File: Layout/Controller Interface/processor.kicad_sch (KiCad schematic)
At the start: 17 parts, among them J1 USB_C_Receptacle_USB2.0, SW2 SW_Push, SW3 SW_Push, SW4 SW_Push, U1 RP2040, U3 W25X40CLSN, Y1 12MHz

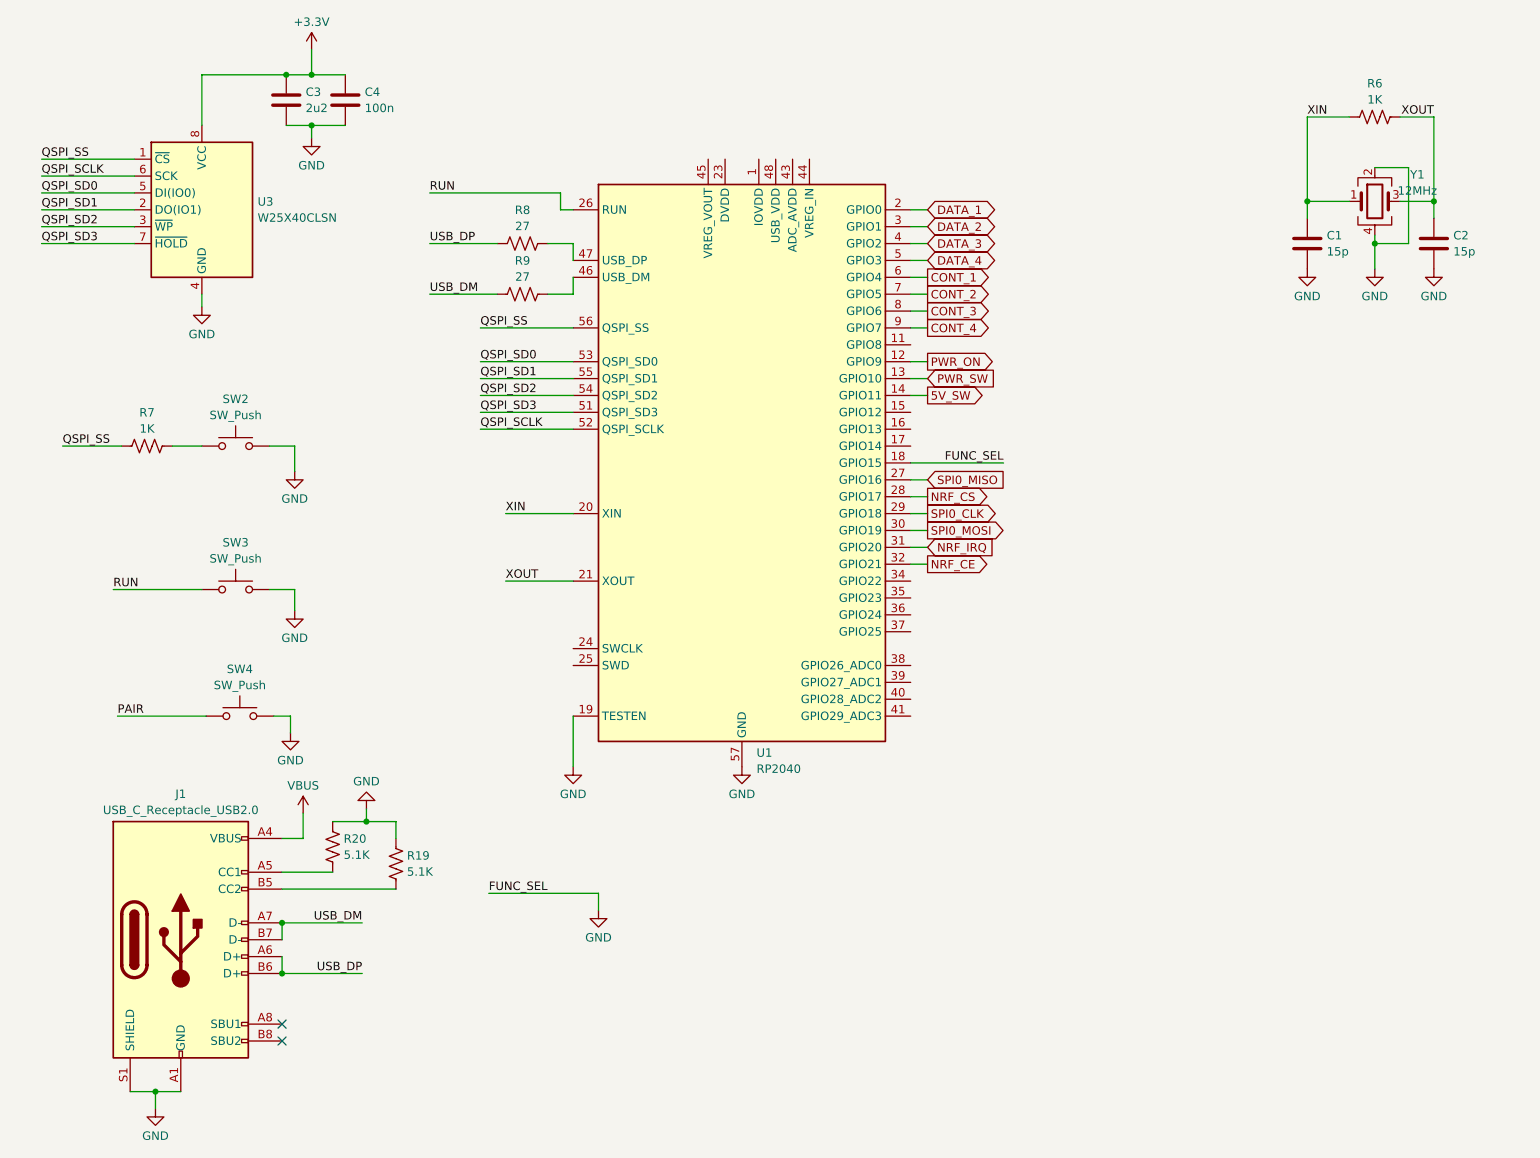
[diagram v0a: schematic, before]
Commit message: Completed schematic and layout
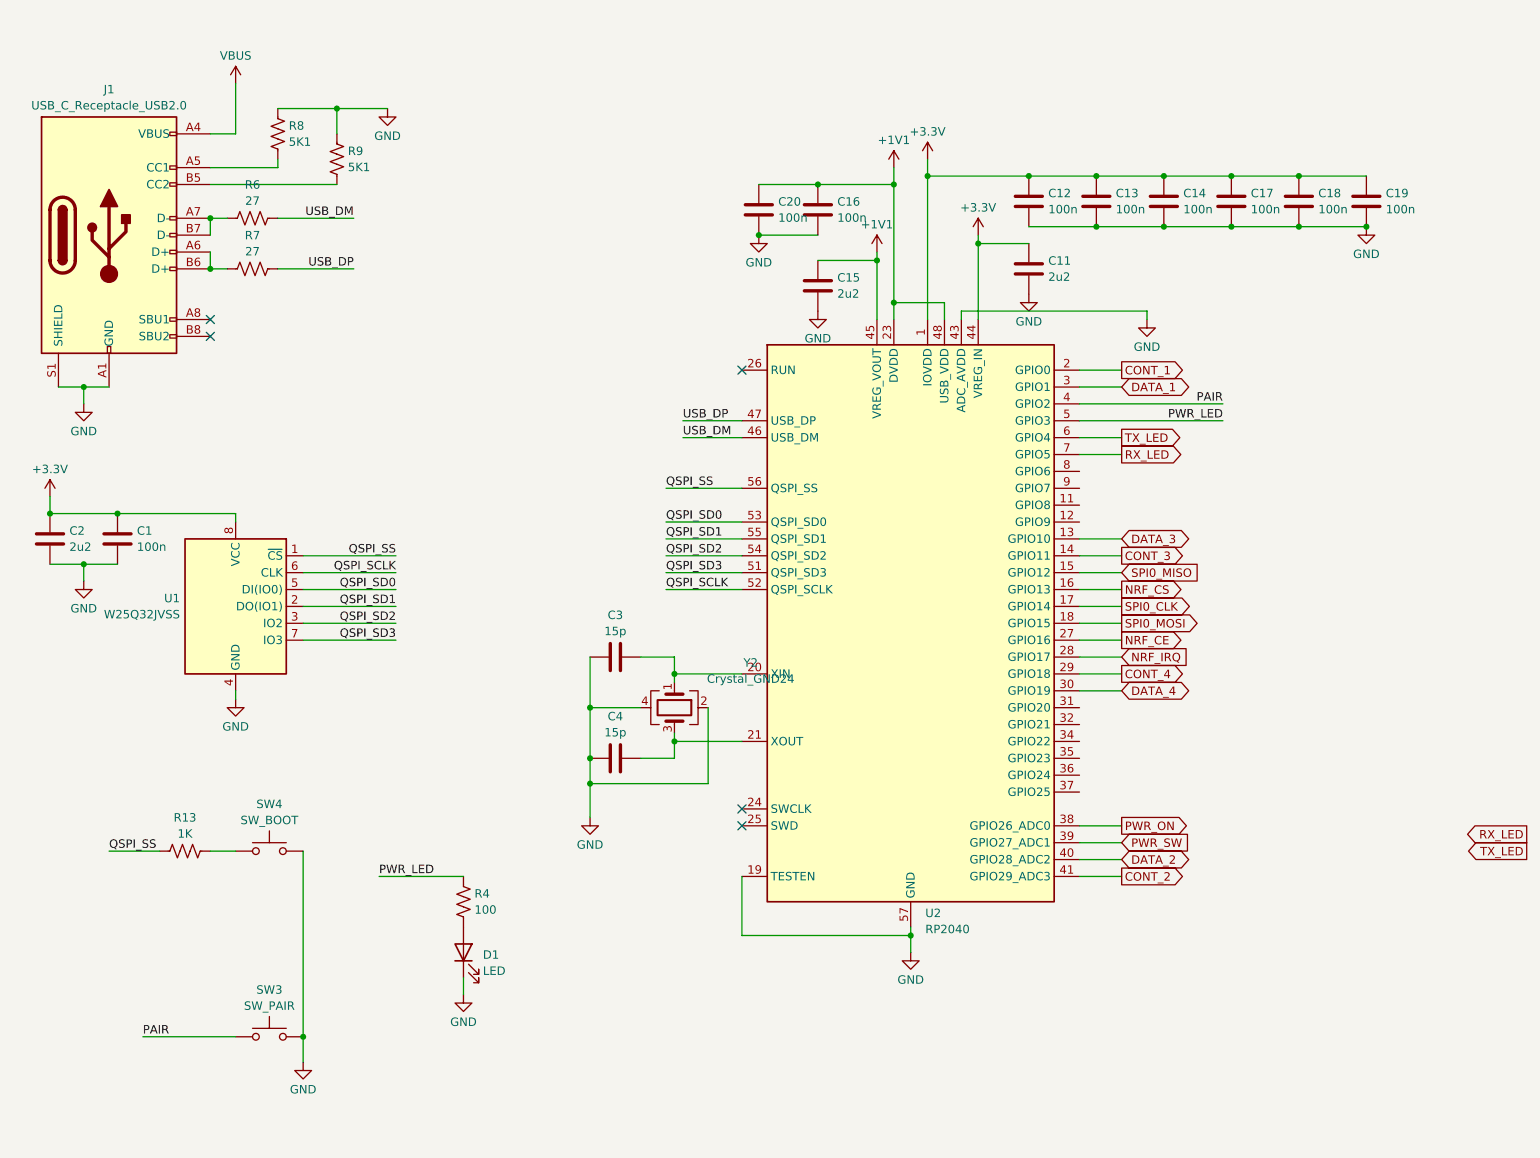
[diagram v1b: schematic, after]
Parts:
- removed R19, R20: 5.1K, Resistor_SMD:R_0805_2012Metric, symbol Device:R_US
- removed SW2: SW_Push, Button_Switch_SMD:SW_SPST_TL3342, symbol Switch:SW_Push
- removed U1: RP2040, Package_DFN_QFN:QFN-56-1EP_7x7mm_P0.4mm_EP3.2x3.2mm, symbol MCU_RaspberryPi:RP2040
- removed U3: W25X40CLSN, Package_SO:SOIC-8_3.9x4.9mm_P1.27mm, symbol Memory_Flash:W25X40CLSN
- removed Y1: 12MHz, Crystal:Crystal_SMD_3225-4Pin_3.2x2.5mm_HandSoldering, symbol Device:Crystal_GND24
- added C11, C15: 2u2, Capacitor_SMD:C_0603_1608Metric, symbol Device:C
- added C12, C13, C14, C16, C17, C18, C19, C20: 100n, Capacitor_SMD:C_0603_1608Metric, symbol Device:C
- added D1: LED, LED_SMD:LED_0805_2012Metric, symbol Device:LED
- added R13: 1K, Resistor_SMD:R_0603_1608Metric, symbol Device:R_US
- added R4: 100, Resistor_SMD:R_0805_2012Metric, symbol Device:R_US
- added U1: W25Q32JVSS, Package_SO:SOIC-8_5.23x5.23mm_P1.27mm, symbol Memory_Flash:W25Q32JVSS
- added U2: RP2040, Package_DFN_QFN:QFN-56-1EP_7x7mm_P0.4mm_EP3.2x3.2mm, symbol MCU_RaspberryPi:RP2040
- added Y2: Crystal_GND24, Crystal:Crystal_SMD_Abracon_ABM8G-4Pin_3.2x2.5mm, symbol Device:Crystal_GND24
- C1: value 15p -> 100n; footprint Capacitor_SMD:C_0805_2012Metric -> Capacitor_SMD:C_0603_1608Metric
- C2: value 15p -> 2u2; footprint Capacitor_SMD:C_0805_2012Metric -> Capacitor_SMD:C_0603_1608Metric
- C3: value 2u2 -> 15p; footprint Capacitor_SMD:C_0805_2012Metric -> Capacitor_SMD:C_0603_1608Metric
- C4: value 100n -> 15p; footprint Capacitor_SMD:C_0805_2012Metric -> Capacitor_SMD:C_0603_1608Metric
- J1: footprint Connector_USB:USB_C_Receptacle_HRO_TYPE-C-31-M-12 -> Connector_USB:USB_C_Receptacle_GCT_USB4105-xx-A_16P_TopMnt_Horizontal
- R6, R7: value 1K -> 27; footprint Resistor_SMD:R_0805_2012Metric -> Resistor_SMD:R_0603_1608Metric
- R8, R9: value 27 -> 5K1; footprint Resistor_SMD:R_0805_2012Metric -> Resistor_SMD:R_0603_1608Metric
- SW3: value SW_Push -> SW_PAIR
- SW4: value SW_Push -> SW_BOOT
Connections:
- net RUN is gone; now on net PAIR: SW3.1
- net +3.3V: now also C1.1, C2.1, C11.1, C12.1, C13.1, C14.1, C17.1, C18.1, C19.1, U1.8 (VCC), U2.1 (IOVDD), U2.10 (IOVDD), U2.22 (IOVDD), U2.33 (IOVDD), U2.42 (IOVDD), U2.44 (VREG_IN), U2.49 (IOVDD); no longer C3.1, C4.1
- net CONT_1: now also U2.2 (GPIO0)
- net CONT_2: now also U2.41 (GPIO29_ADC3)
- net CONT_3: now also U2.14 (GPIO11)
- net CONT_4: now also U2.29 (GPIO18)
- net DATA_1: now also U2.3 (GPIO1)
- net DATA_2: now also U2.40 (GPIO28_ADC2)
- net DATA_3: now also U2.13 (GPIO10)
- net DATA_4: now also U2.30 (GPIO19)
- net GND: now also C4.1, R8.2, R9.2, C11.2, C12.2, C13.2, C14.2, C15.2, C16.2, C17.2, C18.2, C19.2, C20.2, D1.1 (K), U1.4 (GND), U2.19 (TESTEN), U2.43 (ADC_AVDD), U2.57 (GND), Y2.2, Y2.4; no longer C4.2
- net NRF_CE: now also U2.27 (GPIO16)
- net NRF_CS: now also U2.16 (GPIO13)
- net NRF_IRQ: now also U2.28 (GPIO17)
- net PAIR: now also U2.4 (GPIO2); no longer SW4.1
- net PWR_ON: now also U2.38 (GPIO26_ADC0)
- net PWR_SW: now also U2.39 (GPIO27_ADC1)
- net QSPI_SCLK: now also U1.6 (CLK), U2.52 (QSPI_SCLK)
- net QSPI_SD0: now also U1.5 (DI(IO0)), U2.53 (QSPI_SD0)
- net QSPI_SD1: now also U1.2 (DO(IO1)), U2.55 (QSPI_SD1)
- net QSPI_SD2: now also U1.3 (IO2), U2.54 (QSPI_SD2)
- net QSPI_SD3: now also U1.7 (IO3), U2.51 (QSPI_SD3)
- net QSPI_SS: now also R13.1, U1.1 (~{CS}), U2.56 (QSPI_SS); no longer R7.1
- net SPI0_CLK: now also U2.17 (GPIO14)
- net SPI0_MISO: now also U2.15 (GPIO12)
- net SPI0_MOSI: now also U2.18 (GPIO15)
- net USB_DM: now also R6.2, U2.46 (USB_DM); no longer J1.A7 (D-), J1.B7 (D-), R9.1
- net USB_DP: now also R7.2, U2.47 (USB_DP); no longer J1.A6 (D+), J1.B6 (D+), R8.1
- net at J1.A5 (CC1): now also R8.1
- net at J1.B5 (CC2): now also R9.1
- net XIN: no longer names the net of R6.1
- net XIN: now also J1.A7 (D-), J1.B7 (D-); no longer C1.1
- removed net XOUT: C2.1, R6.2
- new net: C3.1, U2.20 (XIN), Y2.1
- new net: C4.2, U2.21 (XOUT), Y2.3
- new net: J1.A6 (D+), J1.B6 (D+), R7.1
- new net: R13.2, SW4.1
- new net: D1.2 (A), R4.2
- new net +1V1: C15.1, C16.1, C20.1, U2.23 (DVDD), U2.45 (VREG_VOUT), U2.48 (USB_VDD), U2.50 (DVDD)
- new net PWR_LED: R4.1, U2.5 (GPIO3)
- new net RX_LED: U2.7 (GPIO5)
- new net TX_LED: U2.6 (GPIO4)
- no-connect marks 2 -> 5
